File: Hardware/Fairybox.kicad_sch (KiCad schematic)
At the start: 80 parts, among them J1 REED, J2 JST B4B-PH-K-S, Q1 SI2302, Q10 C114, Q14 AO3401A, Q15 SI2302, Q16 SI2302, Q2 C114, Q3 C114, Q4 C114, Q5 C114, Q6 C144, Q7 C144, Q8 C114, Q9 C114, U1 ATTINY85, U2 CJ7032

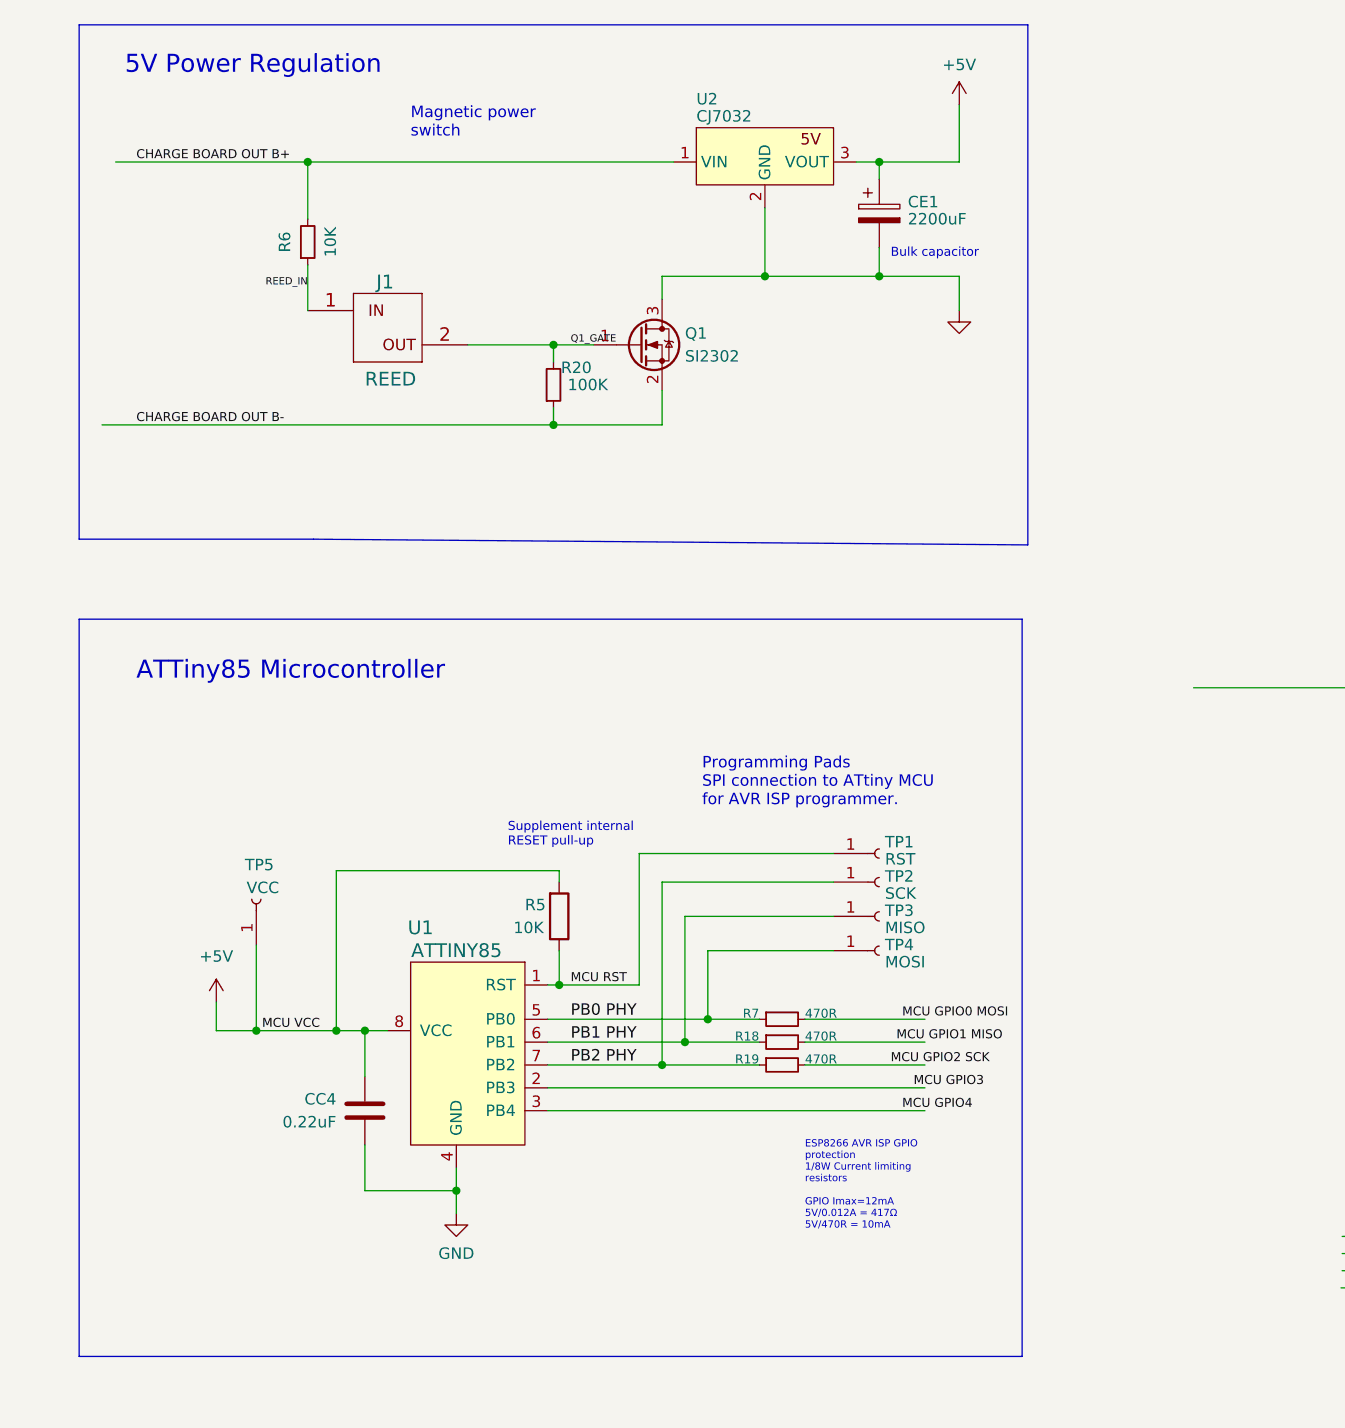
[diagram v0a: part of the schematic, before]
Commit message: not sure
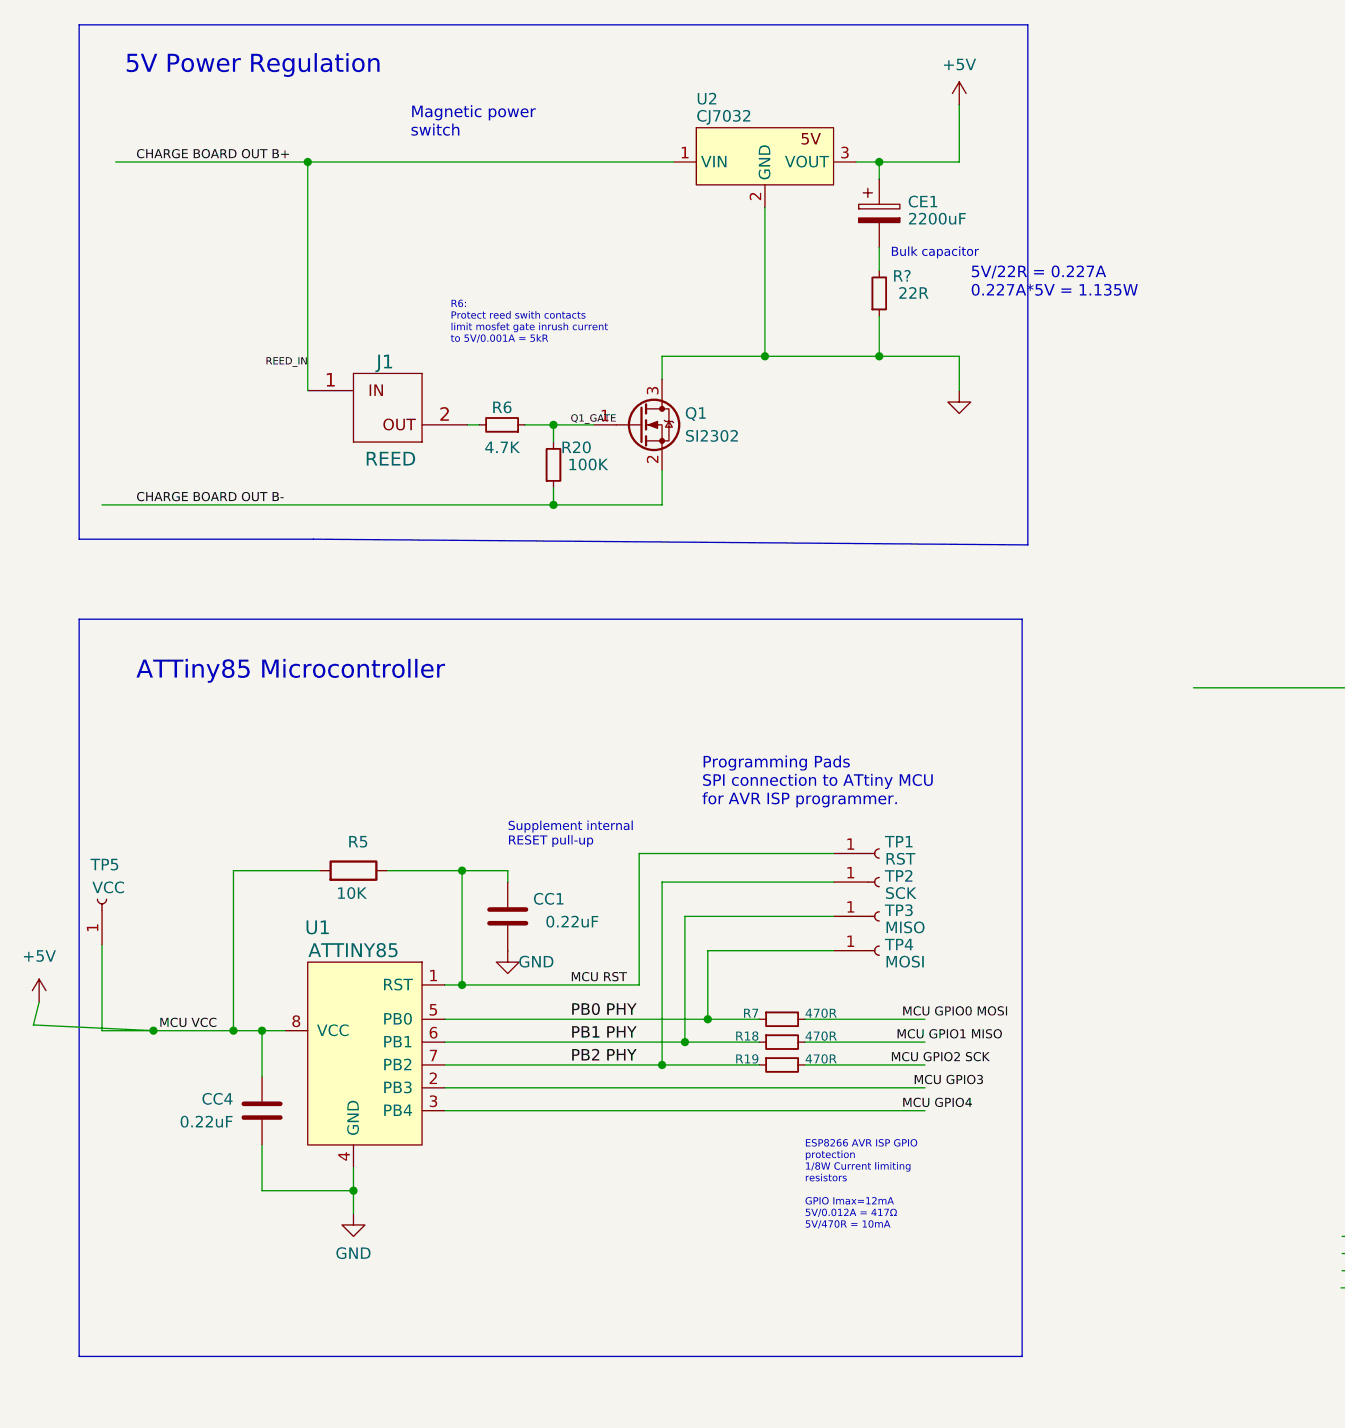
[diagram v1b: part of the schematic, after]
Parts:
- added CC1: 0.22uF, Capacitor_SMD:C_1206_3216Metric, symbol Device:C
- added R?: 22R, Resistor_SMD:R_1206_3216Metric, symbol Device:R_Small
- CC4: footprint Capacitor_THT:C_Disc_D3.0mm_W2.0mm_P2.50mm -> Capacitor_SMD:C_1206_3216Metric
- R6: value 10K -> 4.7K
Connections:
- net CHARGE BOARD OUT B+: now also J1.1; no longer R6.2
- net GND: now also CC1.2, R?.1; no longer CE1.2
- net MCU RST: now also CC1.1
- net Q1_GATE: now also R6.1; no longer J1.2
- removed net REED_IN: J1.1, R6.1
- new net: CE1.2, R?.2
- new net: J1.2, R6.2
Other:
- note added: "5V/22R = 0.227A 0.227A*5V = 1.135W"
- note added: "R6: Protect reed swith contacts limit mosfet gate inrush current to 5V/0.001A = 5kR"
- moved on the sheet: CC4, J1, Q1, R20, R5, R6, TP5, U1
